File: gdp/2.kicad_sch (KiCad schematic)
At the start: 9 parts, among them IC17 MK3881, IC6 74LS85, IC7 PAL16L8

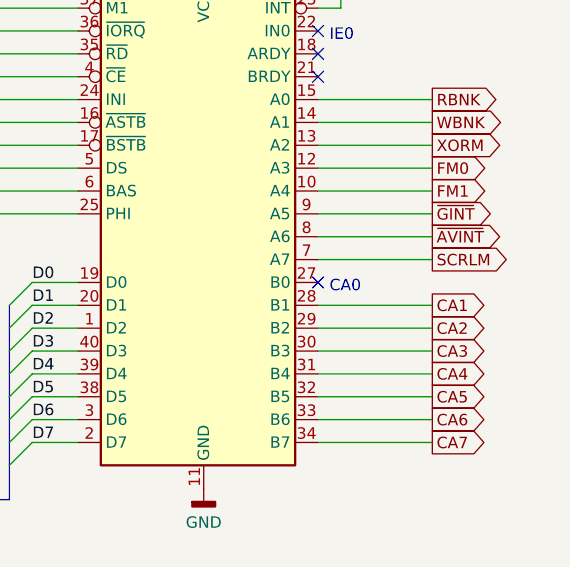
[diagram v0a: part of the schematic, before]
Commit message: Fixes "CA0" issue in schematics
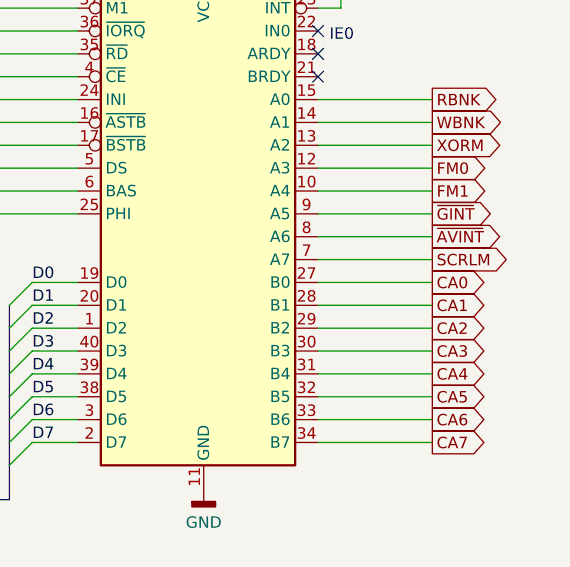
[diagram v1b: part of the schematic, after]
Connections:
- net CA0: now reaches IC17.27 (B0)
- no-connect marks 8 -> 7
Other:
- note removed: "CA0"
